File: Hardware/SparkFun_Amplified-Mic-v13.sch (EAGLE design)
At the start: 16 parts, among them M1 MIC9.7MM, U1 OPA344

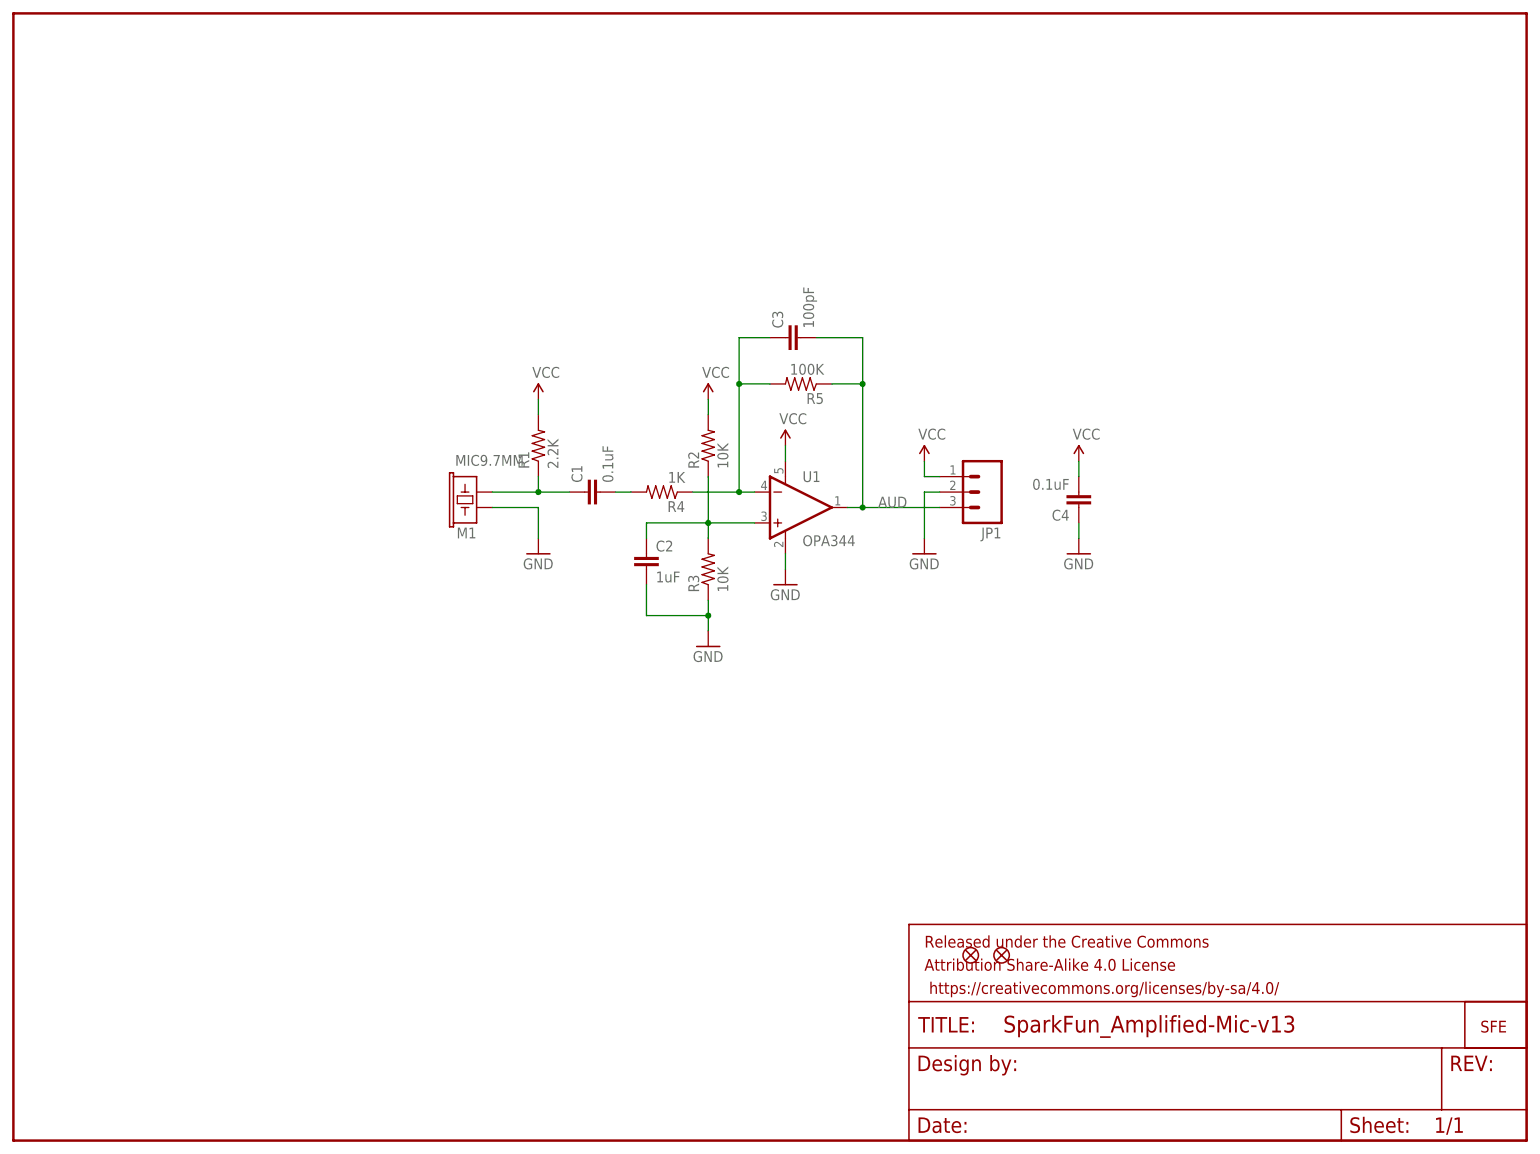
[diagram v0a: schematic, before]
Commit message: few changes made
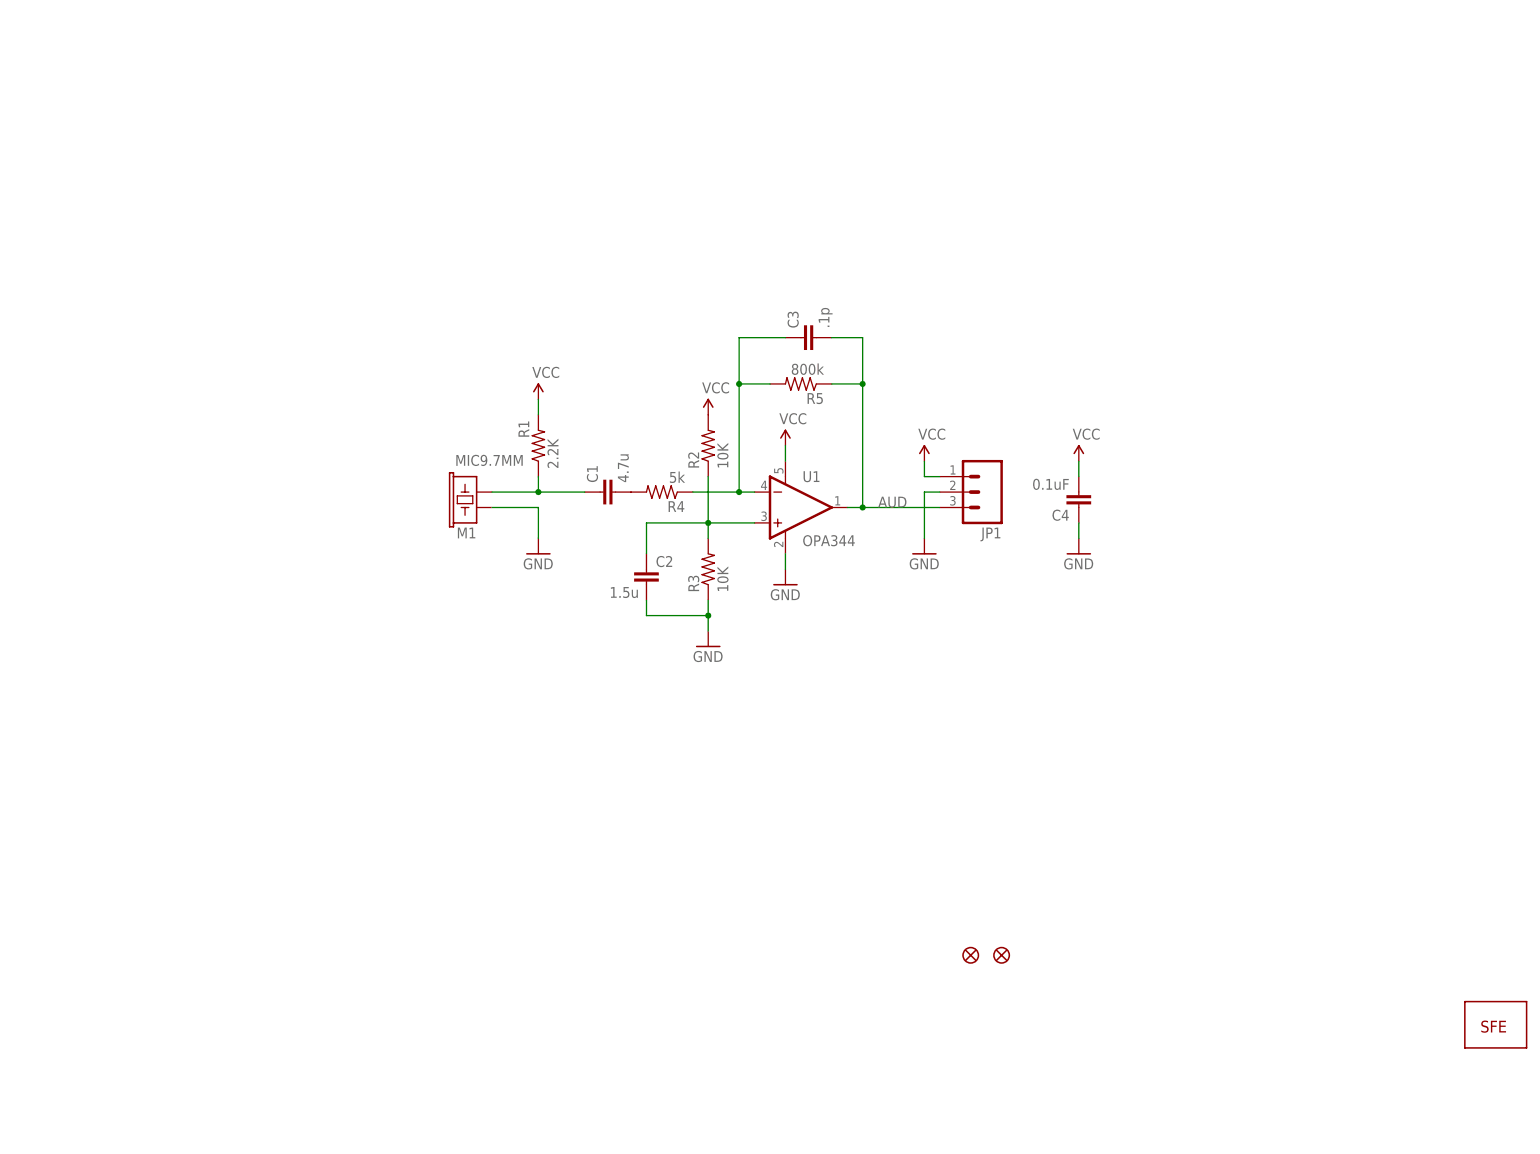
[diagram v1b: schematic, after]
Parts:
- removed FRAME1: FRAME-LETTER, SparkFun-Aesthetics:FRAME-LETTER
- C1: value 0.1uF -> 4.7u; device SparkFun:CAP0402-CAP -> rcl:C-EUC0603
- C2: value 1uF -> 1.5u; device SparkFun:CAP0402-CAP -> rcl:C-EUC0603
- C3: value 100pF -> .1p; device SparkFun:CAP0402-CAP -> rcl:C-EUC0603
- R1: device SparkFun:RESISTOR0402-RES -> rcl:R-US_R0603
- R4: value 1K -> 5k; device SparkFun:RESISTOR0402-RES -> rcl:R-US_R0603
- R5: value 100K -> 800k; device SparkFun:RESISTOR0402-RES -> rcl:R-US_R0603
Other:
- moved on the sheet: C1, C2, C3
